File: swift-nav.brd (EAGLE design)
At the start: 53 x 53 mm, 169 parts, among them J1 SMA_EDGE, J6 ZX62-B-5PA, U1 6SLX9FTG256, U10 MAX2769, U12 PT7M8206B33TA5EX, U13 M25PX80, U2 LTC3407A_DFN, U3 STM32-M-64-LQFP, U4 7Q-16.368MBG-T, U5 SMA_PATCH, U6 93LC56BT-I/OT, U7 FT232HQ, U8 B4050, X4 NX5032GA-12M, X5 CONN_5-2

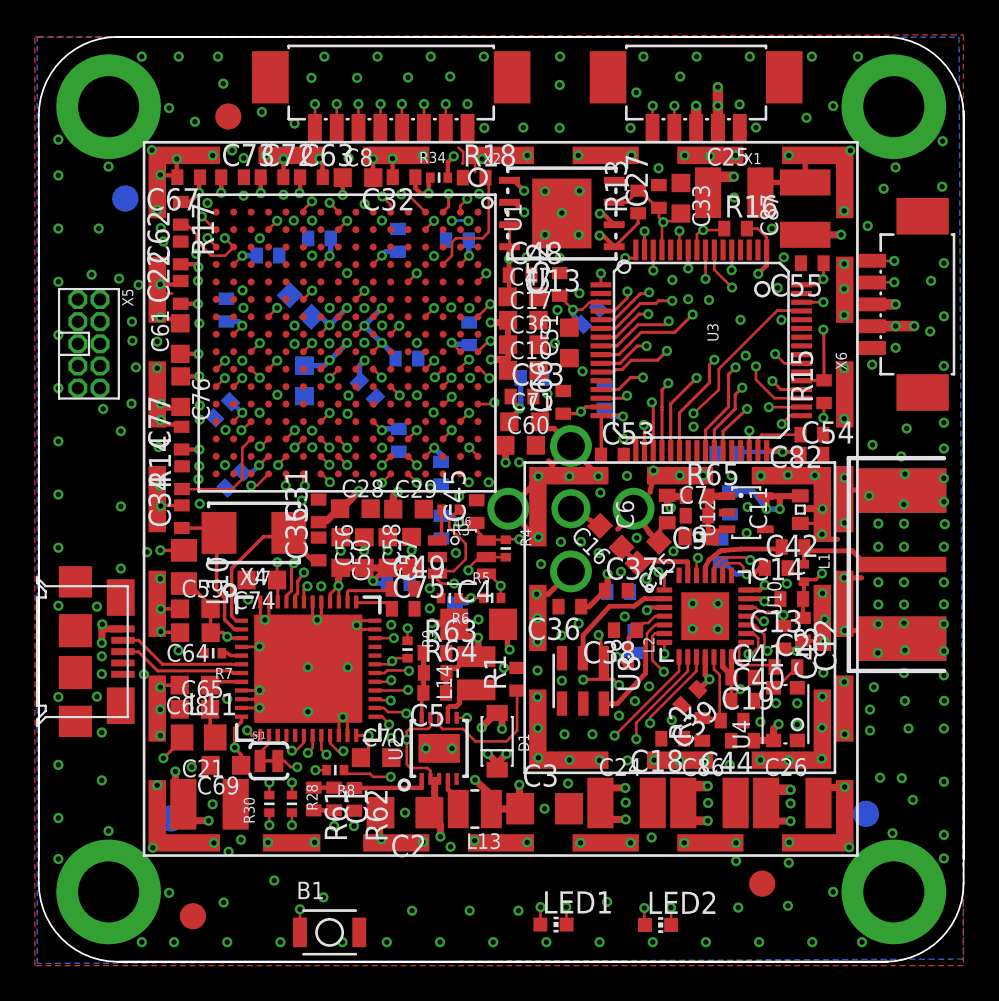
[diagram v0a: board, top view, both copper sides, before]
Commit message: Looots of stuff
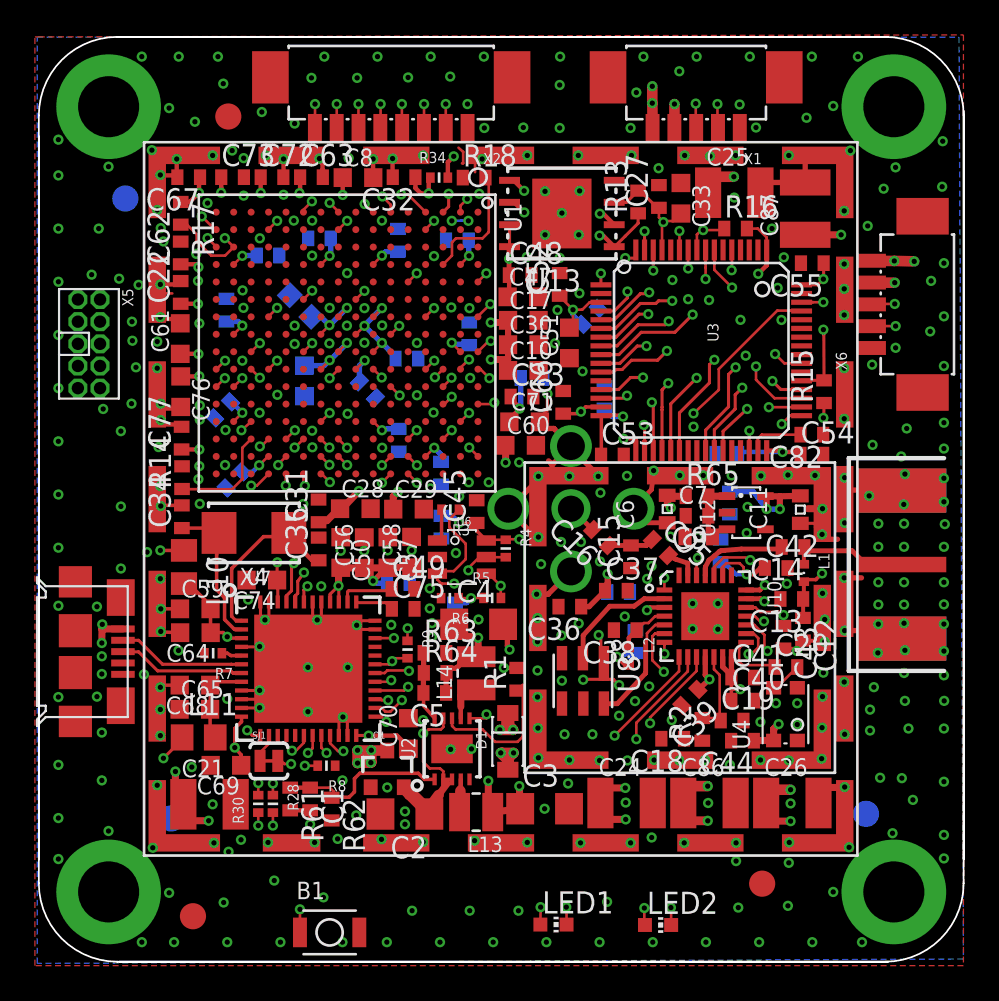
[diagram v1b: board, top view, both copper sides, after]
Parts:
- removed U$1: LOGO, swift-nav:LOGO1
- added C95: 100pF, rcl:C0402
- added Q1: MOSFET-PCHANNELSMD, SparkFun-DiscreteSemi:SOT23-3
- C15, C16: device rcl:C0603K -> rcl:C0402
- moved C70 2.31 mm to (24.6, 16.5), turned to 90 degrees
- moved R62 1.41 mm to (20.2, 12.1)
- moved C1 1.37 mm to (18.9, 12.7)
- moved R61 1.35 mm to (17.8, 12.7)
- moved R28 1.09 mm to (16.8, 12.4)
- moved C15 1.01 mm to (37.3, 26.6), turned to 90 degrees
- moved U2 0.74 mm to (27.1, 15.6)
- moved R30 0.63 mm to (16.0, 12.4)
- moved D1 0.61 mm to (30.3, 16.0), turned to 90 degrees
- moved C16 0.59 mm to (35.6, 27.7)
- moved R8 0.57 mm to (19.9, 14.6)
- moved L13 0.19 mm to (28.5, 12.0)
- moved C2 0.08 mm to (24.4, 11.9)
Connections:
- new net N$18: C2.1, Q1.2, R1.2, U2.2, U2.3, U2.6, U2.9
- new net N$35: C15.2, C16.1, C95.1
- net GND: now also Q1.1
- net N$11: now also C95.2; no longer C15.2, C16.1
- net UART1_RX: now also X6.2; no longer X6.5
- net UART1_TX: now also X6.3; no longer X6.4
- net UART3_RX: now also X1.2; no longer X1.5
- net UART3_TX: now also X1.3; no longer X1.4
- net V+: now also Q1.3, X1.5, X6.5; no longer C2.1, R1.2, U2.2, U2.3, U2.6, U2.9, X1.2, X6.2
- net VCCIO: now also X1.4, X6.4; no longer X1.3, X6.3
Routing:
- net N$18: track 0.00 -> 20.4 mm, vias 0 -> 3
- net GND: track 97.8 -> 91.5 mm, vias 405 -> 404
- net UART3_RX: track 26.9 -> 22.2 mm
- net UART1_RX: track 19.3 -> 15.2 mm
- net N$53: track 6.71 -> 10.1 mm
- net V+: track 134.1 -> 137.3 mm, vias 13 -> 12
- net N$11: track 5.02 -> 1.89 mm
- net N$35: track 0.00 -> 2.65 mm
- net VCCIO: track 164.8 -> 167.1 mm
- net V_USB: track 115.0 -> 117.0 mm, vias 6 -> 8
- net N$55: track 23.9 -> 25.5 mm
- net UART3_TX: track 25.3 -> 23.8 mm
- net N$24: track 19.4 -> 20.6 mm
- net FTDI_NRST: track 110.2 -> 109.5 mm
- net UART6_TX: track 52.1 -> 51.3 mm
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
